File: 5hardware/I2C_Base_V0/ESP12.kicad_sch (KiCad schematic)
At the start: 43 parts, among them J1 Conn_01x39_Socket, J4 Conn_01x39_Socket, P2 S4B-PH-SM4-TB, SW1 SW_Push, SW2 SW_Push, SW5 RotaryEncoder, U10 ESP-12F, U14 Lolin_Base, U2 ESP32-C3-WROOM-02, U9 E18-MS1-PCB

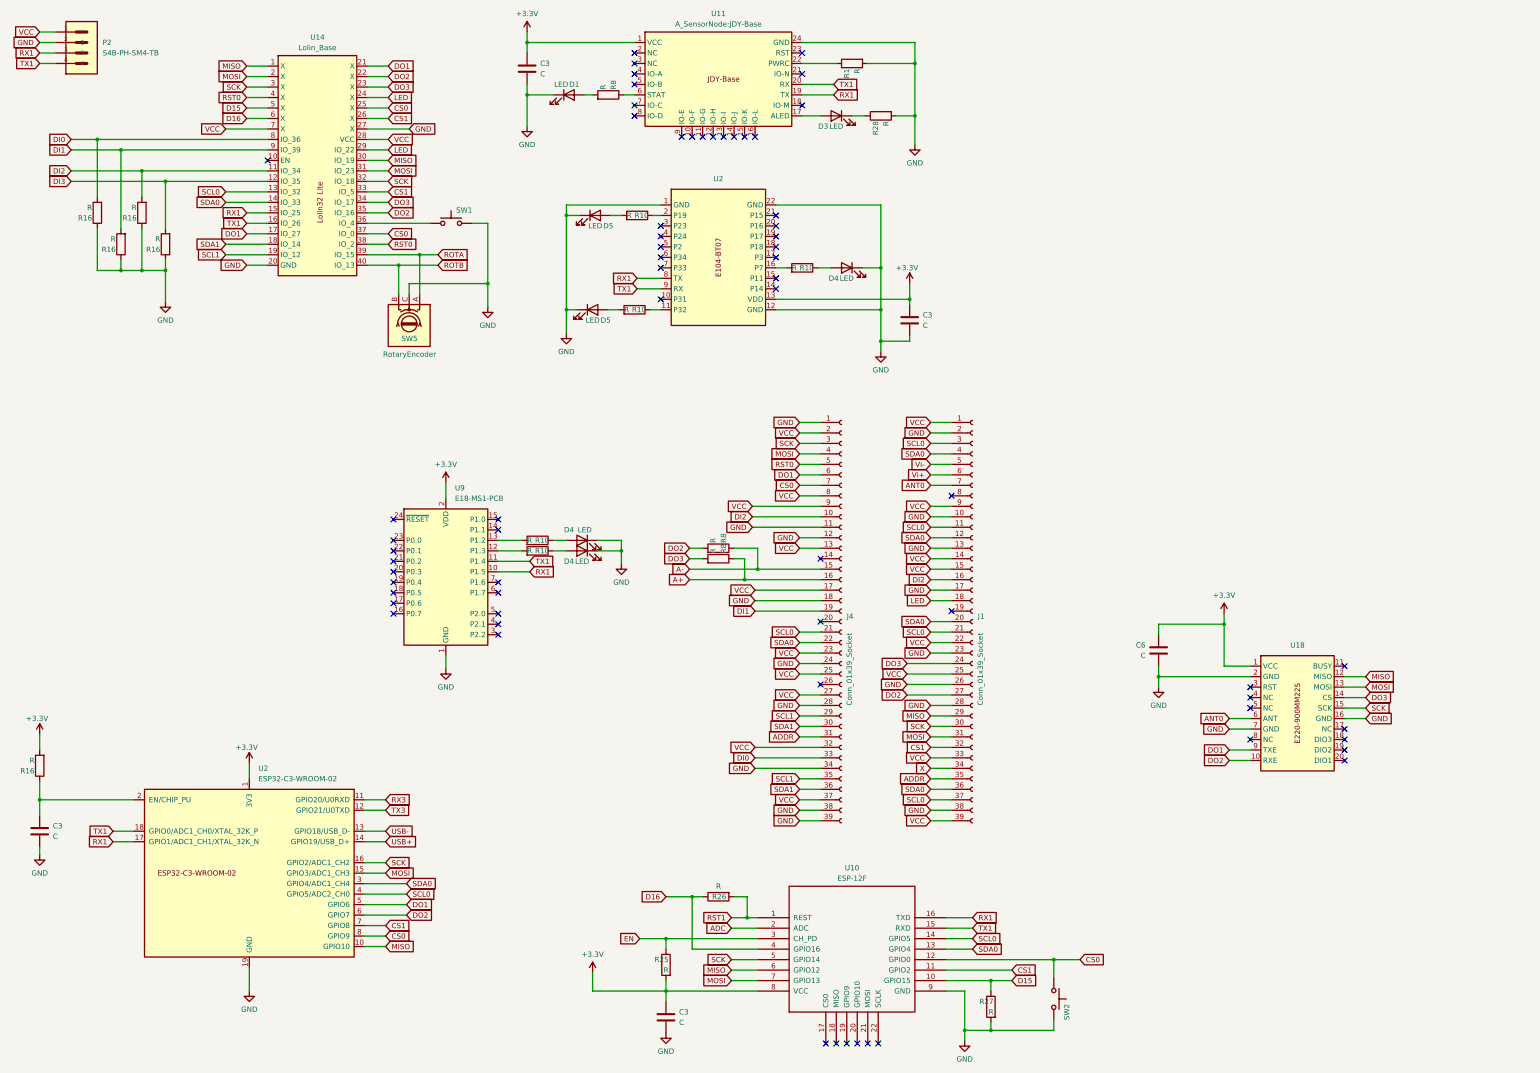
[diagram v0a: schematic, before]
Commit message: update PCB.
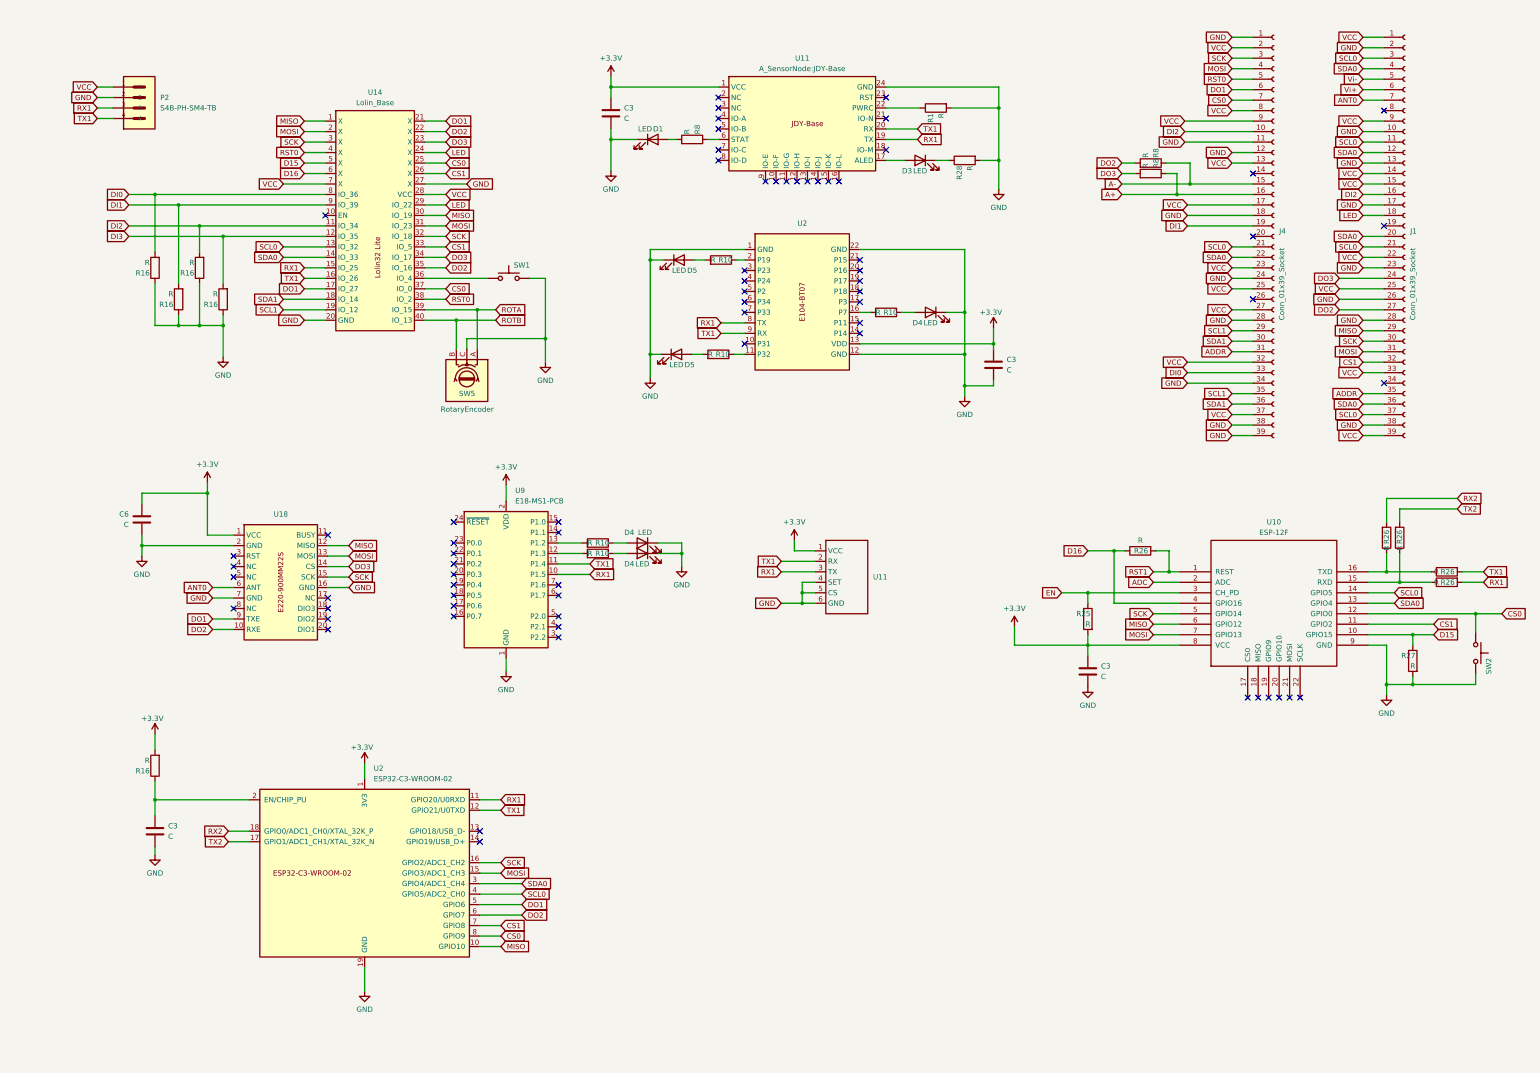
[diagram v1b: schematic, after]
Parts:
- added R26 (x4): R, Resistor_SMD:R_0805_2012Metric, symbol Device:R
- added U11: ~, A_SensorNode:JDY-41, symbol A_SensorNode:JDY-41
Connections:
- net RX3 is gone; now on net RX1: U2.11 (GPIO20/U0RXD)
- net TX3 is gone; now on net TX1: U2.12 (GPIO21/U0TXD)
- net +3.3V: now also U11.1 (VCC)
- net GND: now also U11.4 (SET), U11.5 (CS), U11.6 (GND)
- net RX1: now also R26.2, U11.3 (TX); no longer U10.16 (TXD), U2.17 (GPIO1/ADC1_CH1/XTAL_32K_N)
- net TX1: now also R26.2, U11.2 (RX); no longer U10.15 (RXD), U2.18 (GPIO0/ADC1_CH0/XTAL_32K_P)
- net USB+: no longer names the net of U2.14 (GPIO19/USB_D+)
- net USB-: no longer names the net of U2.13 (GPIO18/USB_D-)
- net X: no longer names the net of J1.34 (Pin_34)
- new net: R26.1, R26.1, U10.15 (RXD)
- new net: R26.1, R26.1, U10.16 (TXD)
- new net RX2: R26.2, U2.18 (GPIO0/ADC1_CH0/XTAL_32K_P)
- new net TX2: R26.2, U2.17 (GPIO1/ADC1_CH1/XTAL_32K_N)
- no-connect marks 67 -> 70
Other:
- moved on the sheet: C3, C6, D1, D3, D4, D5, J1, J4, P2, R1, R10, R16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
